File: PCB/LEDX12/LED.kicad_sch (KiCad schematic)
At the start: 33 parts, among them J1 Conn_01x03, J2 TC2030-USB-NL-DS, P1 Square, P2 Square, P3 Square, P4 Square, U1 TPS562246, U2 ESP32-S3-MINI-1, U3 ICS43434_MEMS_Mic

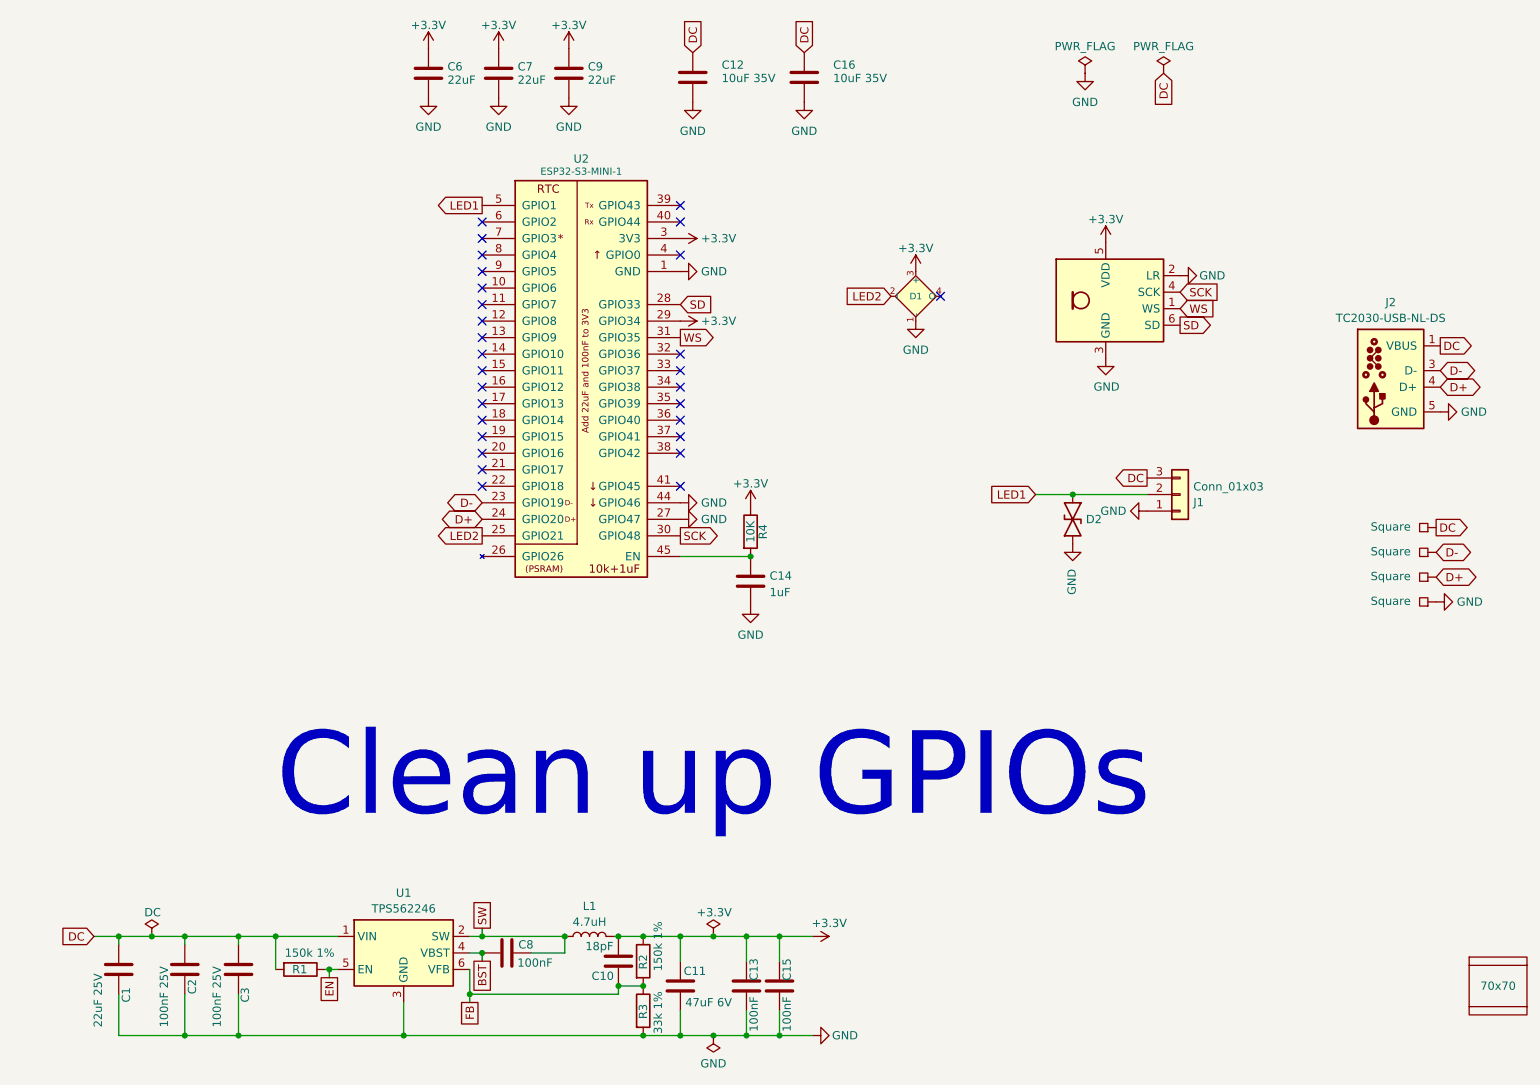
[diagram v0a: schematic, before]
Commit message: Library update
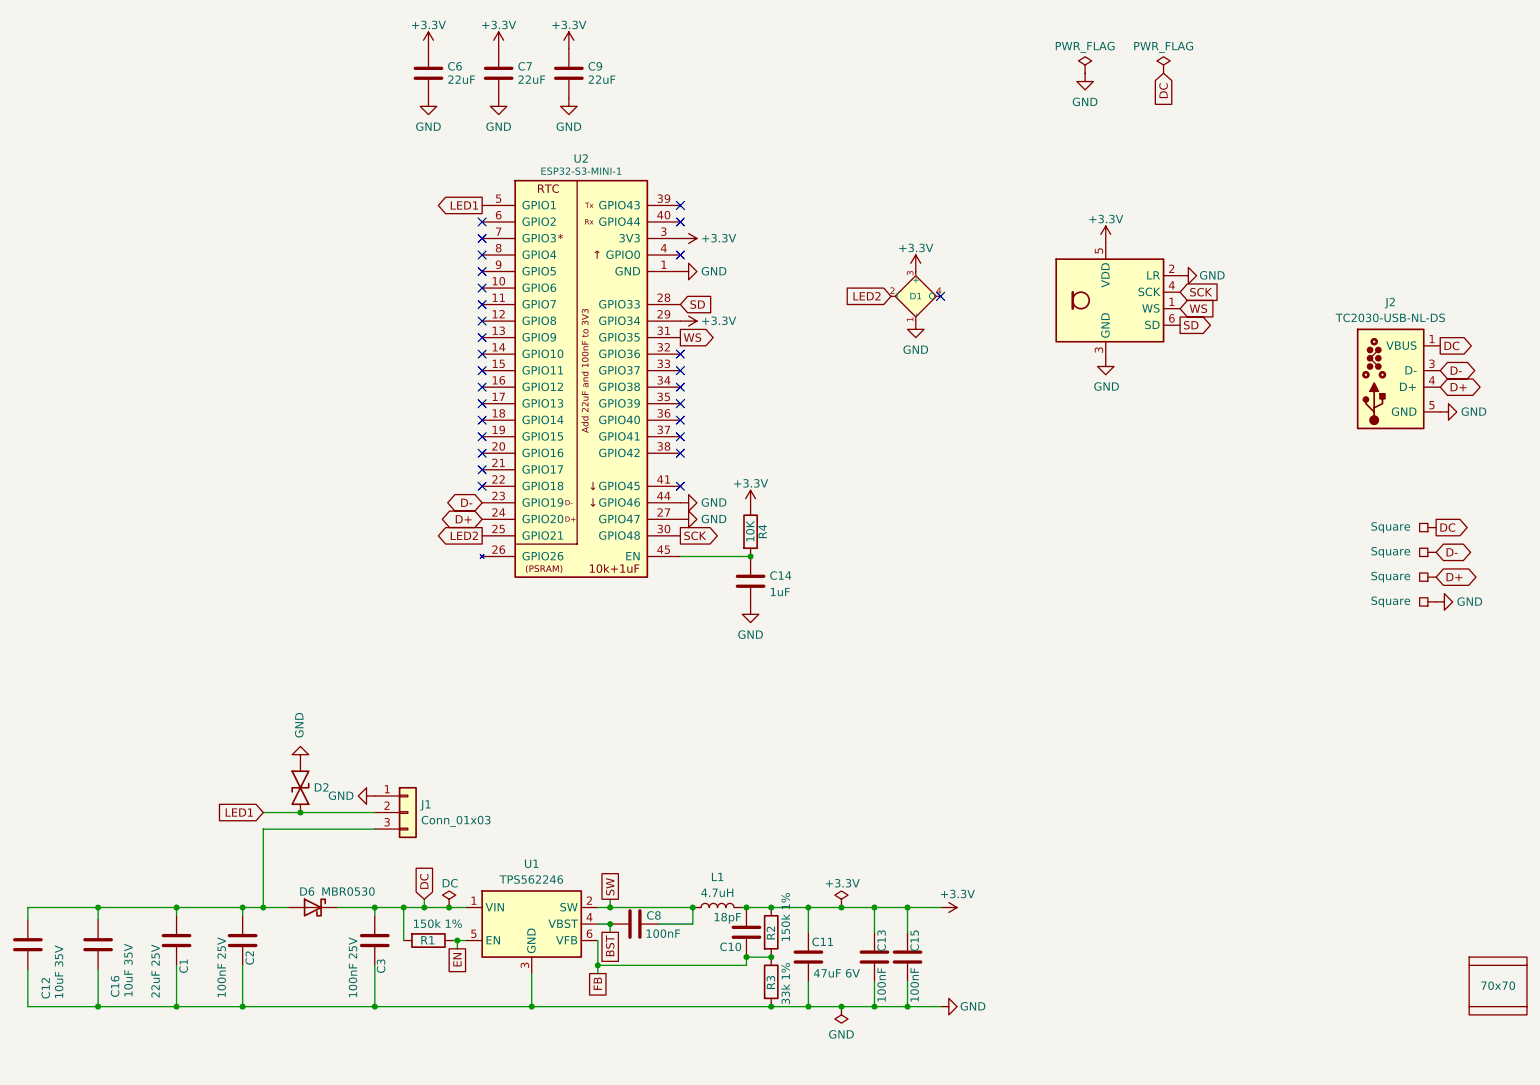
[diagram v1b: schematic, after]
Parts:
- added D6: MBR0530, RevK:D_SOD-123, symbol Diode:1N5819
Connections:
- net DC: now also D6.1 (K); no longer C1.1, C12.1, C16.1, C2.1, J1.3 (Pin_3)
- new net: C1.1, C12.1, C16.1, C2.1, D6.2 (A), J1.3 (Pin_3)
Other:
- note removed: "Clean up GPIOs"
- moved on the sheet: C1, C10, C11, C12, C13, C15, C16, C2, C3, C8, D2, J1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
